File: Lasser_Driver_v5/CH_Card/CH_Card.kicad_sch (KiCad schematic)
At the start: 150 parts, among them J1 DIN41612_M_universal, Q13 IRL540N, Q14 IRF9540N, Q17 IRL540N, Q18 IRF9540N, Q19 DMN3404L, U101 AD5696R, U102 ADS1115, U103 PCA9538, U104 ADG419BRM, U105 ADG419BRM, U17 OPA192IDBVR, U19 OPA192IDBVR, U21 OPA551U, U22 OPA192IDBVR, U24 OPA192IDBVR, U26 ADG419BRM, U28 INA828, U32 INA828

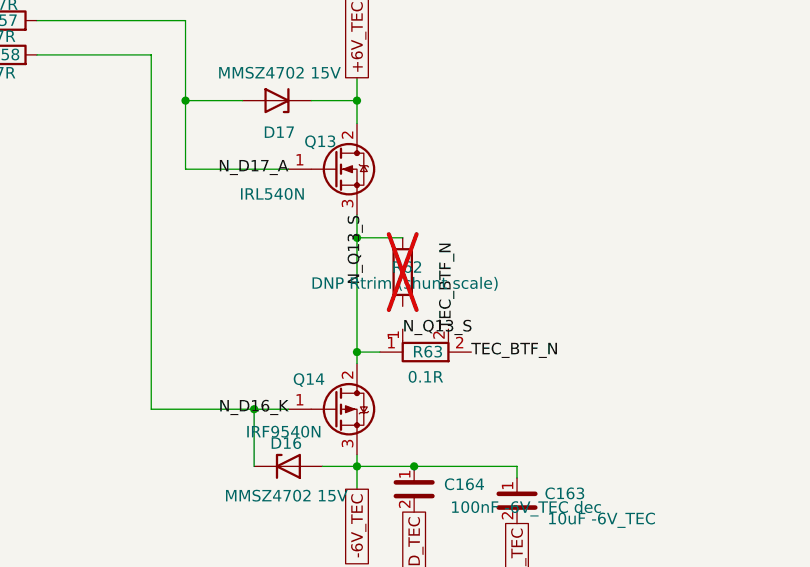
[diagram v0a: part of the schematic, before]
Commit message: Working on the CH pcb layout and routing.
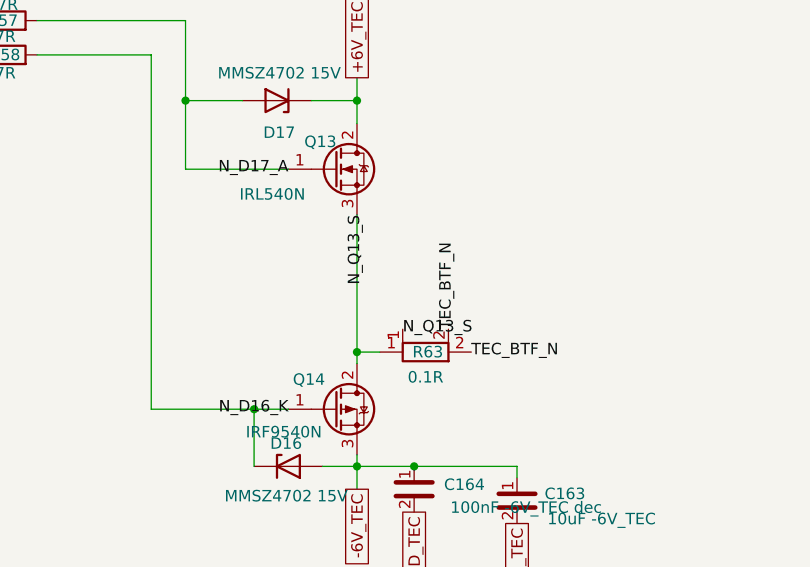
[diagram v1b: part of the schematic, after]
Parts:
- removed R62: DNP Rtrim (shunt scale), Resistor_SMD:R_0805_2012Metric_Pad1.20x1.40mm_HandSolder, symbol Device:R
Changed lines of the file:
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@@
 	)
 	(junction
-		(at 382.27 212.09)
-		(diameter 0)
-		(color 0 0 0 0)
-	)
-	(junction
 		(at 82.55 210.82)
 		(diameter 0)
@@
 	(wire
 		(pts
-			(xy 382.27 209.55) (xy 382.27 212.09)
-		)
-		(stroke
-			(width 0)
-			(type default)
-		)
-	)
-	(wire
-		(pts
 			(xy 143.51 207.01) (xy 143.51 208.28)
 		)
@@
 	(wire
 		(pts
-			(xy 382.27 212.09) (xy 387.35 212.09)
-		)
-		(stroke
-			(width 0)
-			(type default)
-		)
-	)
-	(wire
-		(pts
 			(xy 388.62 128.27) (xy 388.62 130.81)
 		)
@@
 	(wire
 		(pts
-			(xy 382.27 212.09) (xy 382.27 224.79)
+			(xy 382.27 209.55) (xy 382.27 224.79)
 		)
 		(stroke
@@
 		(pin "7"
 		)
+		(pin "8"
+		)
+		(pin "5"
+		)
+		(pin "1"
+		)
 		(instances
 			(project "CH_Card"
@@
 	)
 	(symbol
-		(lib_id "Device:R")
-		(at 387.35 215.9 0)
-		(unit 1)
-		(body_style 1)
-		(exclude_from_sim no)
-		(in_bom yes)
-		(on_board yes)
-		(in_pos_files yes)
-		(dnp yes)
-		(property "Reference" "R62"
-			(at 387.858 215.392 0)
-			(show_name no)
-			(do_not_autoplace no)
-			(effects
-				(font
-					(size 1.27 1.27)
-				)
-			)
-		)
-		(property "Value" "DNP Rtrim (shunt scale)"
-			(at 387.604 217.17 0)
-			(show_name no)
-			(do_not_autoplace no)
-			(effects
-				(font
-					(size 1.27 1.27)
-				)
-			)
-		)
-		(property "Footprint" "Resistor_SMD:R_0805_2012Metric_Pad1.20x1.40mm_HandSolder"
-			(at 387.35 215.9 0)
-			(hide yes)
-			(show_name no)
-			(do_not_autoplace no)
-			(effects
-				(font
-					(size 1.27 1.27)
-				)
-			)
-		)
-		(property "Datasheet" ""
-			(at 387.35 215.9 0)
-			(hide yes)
-			(show_name no)
-			(do_not_autoplace no)
-			(effects
-				(font
-					(size 1.27 1.27)
-				)
-			)
-		)
-		(property "Description" ""
-			(at 387.35 215.9 0)
-			(show_name no)
-			(do_not_autoplace no)
-			(effects
-				(font
-					(size 1.27 1.27)
-				)
-			)
-		)
-		(pin "1"
-		)
-		(pin "2"
-		)
-		(instances
-			(project "CH_Card"
-				(path "/2abe37a0-24c0-47ee-a2b1-3dcf608486c0"
-					(reference "R62")
-					(unit 1)
-				)
-			)
-		)
-	)
-	(symbol
 		(lib_id "Device:C")
 		(at 54.61 182.88 0)
@@
 		)
 		(property "Footprint" "Package_SO:SOIC-8_3.9x4.9mm_P1.27mm"
-			(at 542.29 53.34 0)
+			(at 545.338 36.576 0)
 			(hide yes)
 			(show_name no)
@@
 		(pin "3"
 		)
+		(pin "1"
+		)
+		(pin "8"
+		)
+		(pin "5"
+		)
 		(instances
